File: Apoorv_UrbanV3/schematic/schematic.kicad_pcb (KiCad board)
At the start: 2 copper layers, 126 x 72 mm, 15 parts

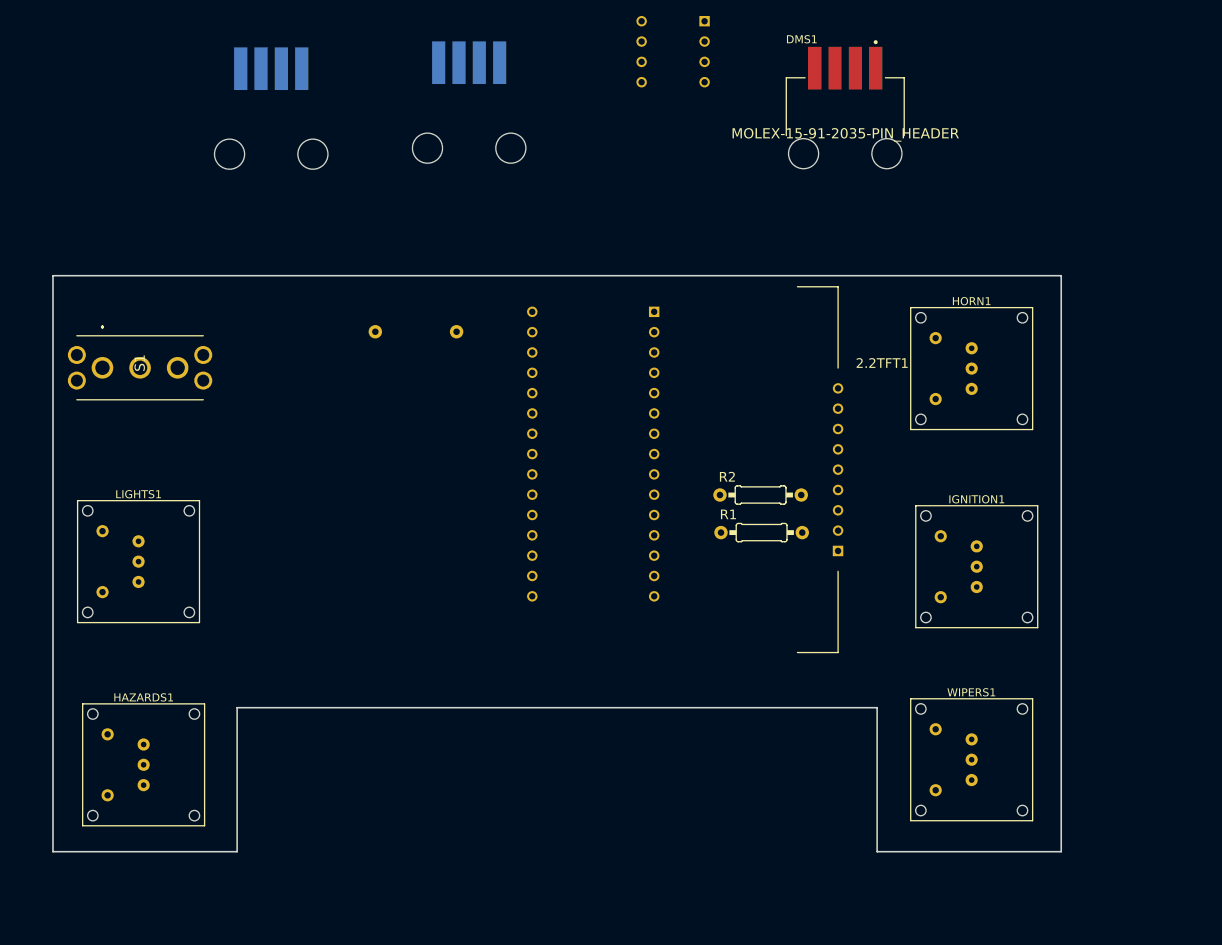
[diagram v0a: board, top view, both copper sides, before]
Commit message: ALMOST DONE, ROUTING LEFT
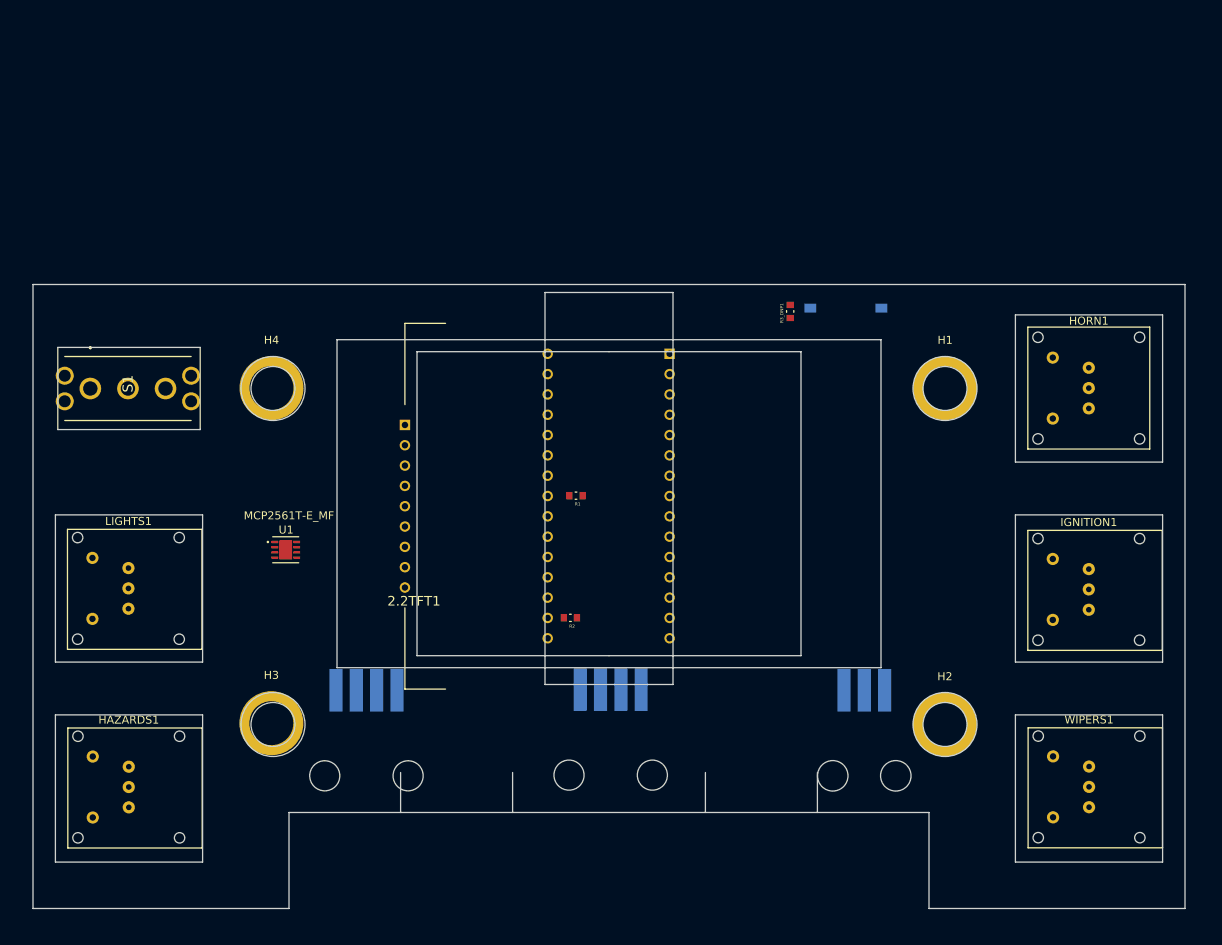
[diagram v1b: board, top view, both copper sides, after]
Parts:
- removed TRANSCEIVER1: MCP2561-THROUGH, schematic:DIP787W46P254L927H533Q8
- added H1: MountingHole_Pad, MountingHole:MountingHole_5mm_Pad, F.Cu at (196.1, 68.5)
- added H2: MountingHole_Pad, MountingHole:MountingHole_5mm_Pad, F.Cu at (196.0, 110.5)
- added H3: MountingHole_Pad, MountingHole:MountingHole_5mm_Pad, F.Cu at (111.9, 110.4)
- added H4: MountingHole_Pad, MountingHole:MountingHole_5mm_Pad, F.Cu at (111.9, 68.5)
- added S2: DS04-254-2-01BK-SMT, dip_swtich_1pos:SW_DS04-254-2-01BK-SMT, B.Cu at (183.7, 58.5)
- added U1: MCP2561T-E_MF, MCP2561:MCP2561T-E&slash_MF, F.Cu at (113.6, 88.7)
- DMS1: footprint eec:Molex-15-91-2045-0-0-0 -> 15-91-2035:15912035; moved to B.Cu
- R1, R2: footprint schematic:0207_10 -> 10k_resistor:RESC1608X55N
- R3_DNP1: footprint schematic:0207_10 -> 10k_resistor:RESC1608X55N; moved to F.Cu
- moved MAINPLUG1 88.5 mm to (154.3, 114.4)
- moved DMS1 80.3 mm to (186.0, 116.9), turned to 180 degrees
- moved BRAKE+THROTTLE1 79.5 mm to (123.7, 114.4)
- moved 2.2TFT1 49.3 mm to (131.1, 83.2), turned to 0 degrees
- moved R3_DNP1 46.8 mm to (176.7, 58.9), turned to 90 degrees
- moved R2 28.3 mm to (149.2, 97.2), turned to 180 degrees
- moved R1 23.7 mm to (149.9, 81.9), turned to 180 degrees
- moved WIPERS1 15.1 mm to (214.1, 113.2)
- moved HORN1 14.8 mm to (214.0, 63.4)
- moved IGNITION1 14.3 mm to (214.0, 88.6)
- moved STM32L432 5.59 mm to (154.0, 70.5)
- moved LIGHTS1 3.58 mm to (94.0, 88.4)
- moved HAZARDS1 3.34 mm to (94.0, 113.3)
- moved S1 3.00 mm to (89.2, 68.5)
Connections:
- 2.2TFT1 pad 4: +5V -> Net-(2.2TFT1-Pad4)
- 2.2TFT1 pad 5: Net-(2.2TFT1-Pad5) -> +5V
- R1 pad 2: +5V -> Net-(2.2TFT1-Pad4)
- R3_DNP1 pad 2: Net-(MAINPLUG1-Pad2) -> Net-(R3_DNP1-Pad2)
- STM32L432 pad 22: Net-(2.2TFT1-Pad5) -> +5V
- STM32L432 pad 23: +5V -> Net-(2.2TFT1-Pad4)
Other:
- board size 126 x 72 mm -> 144 x 78 mm
- board text removed: "ELEC_URB_STEERING_R3"
- board text removed: "SEMA"

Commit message: V3 done design review pending
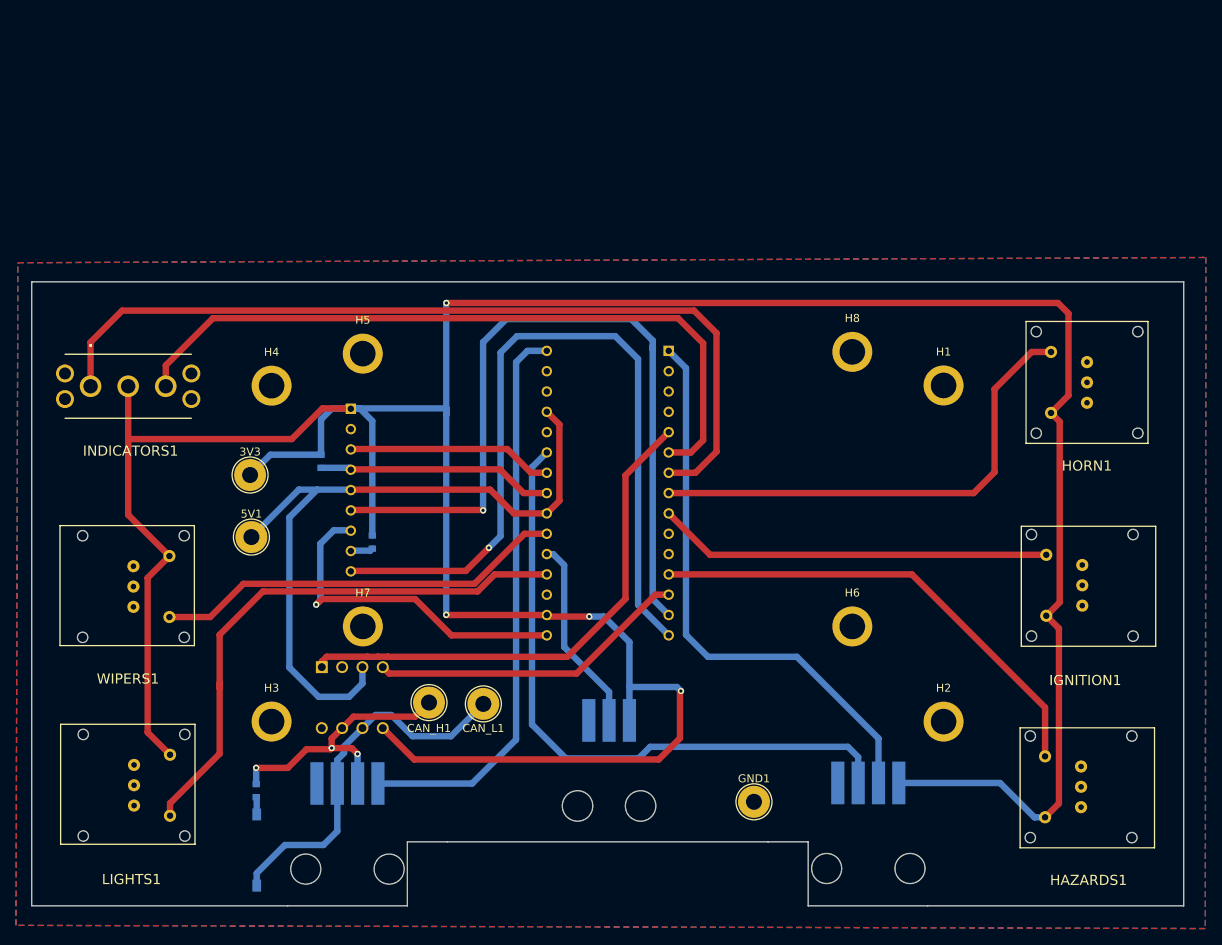
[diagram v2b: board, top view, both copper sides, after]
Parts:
- removed 2.2TFT1: 2.2TFT, schematic:2.2TFT
- removed U1: MCP2561T-E_MF, MCP2561:MCP2561T-E&slash_MF
- added 3V3: TestPoint, TestPoint:TestPoint_THTPad_D4.0mm_Drill2.0mm, F.Cu at (109.2, 79.3)
- added 5V1: TestPoint, TestPoint:TestPoint_THTPad_D4.0mm_Drill2.0mm, F.Cu at (109.4, 87.1)
- added CAN_H1: TestPoint, TestPoint:TestPoint_THTPad_D4.0mm_Drill2.0mm, F.Cu at (131.6, 107.8)
- added CAN_L1: TestPoint, TestPoint:TestPoint_THTPad_D4.0mm_Drill2.0mm, F.Cu at (138.4, 108.0)
- added CAN_TRNSVR1: `, footprints:MCP2562FD-H&slash_P, B.Cu at (118.2, 103.4)
- added GND1: TestPoint, TestPoint:TestPoint_THTPad_D4.0mm_Drill2.0mm, F.Cu at (172.2, 120.2)
- added H5: MountingHole_Pad, MountingHole:MountingHole_3.2mm_M3_Pad, F.Cu at (123.3, 64.2)
- added H6: MountingHole_Pad, MountingHole:MountingHole_3.2mm_M3_Pad, F.Cu at (184.5, 98.3)
- added H7: MountingHole_Pad, MountingHole:MountingHole_3.2mm_M3_Pad, F.Cu at (123.3, 98.3)
- added H8: MountingHole_Pad, MountingHole:MountingHole_3.2mm_M3_Pad, F.Cu at (184.5, 63.9)
- added LCD1: 2.2TFT, schematic:2.2TFT, F.Cu at (124.3, 81.2)
- BRAKE+THROTTLE1: value MOLEX-15-91-2045-PIN_HEADER -> `
- DMS1: value MOLEX-15-91-2035-PIN_HEADER -> `
- H1, H2, H3, H4: footprint MountingHole:MountingHole_5mm_Pad -> MountingHole:MountingHole_3.2mm_M3_Pad
- HAZARDS1, IGNITION1, LIGHTS1, WIPERS1: value LP11EE1NCSYG -> `
- HORN1: value LP11OA1TCSYY -> `
- INDICATORS1: renamed from S1; value M2013TXG13-DA -> `
- R1, R2: moved to B.Cu
- R_CAN1: renamed from R3_DNP1; moved to B.Cu
- S_CAN1: renamed from S2; value DS04-254-2-01BK-SMT -> ~
- moved WIPERS1 120.4 mm to (94.6, 98.4), turned to 180 degrees
- moved HAZARDS1 119.0 mm to (213.1, 113.2)
- moved S_CAN1 100.1 mm to (110.0, 126.2), turned to 270 degrees
- moved R_CAN1 89.7 mm to (110.0, 118.8), turned to 270 degrees
- moved BRAKE+THROTTLE1 63.8 mm to (186.5, 126.0)
- moved MAINPLUG1 34.9 mm to (121.4, 126.1)
- moved LIGHTS1 34.8 mm to (94.7, 123.2), turned to 180 degrees
- moved R1 32.2 mm to (118.1, 77.6), turned to 270 degrees
- moved DMS1 32.1 mm to (154.1, 120.7)
- moved R2 26.5 mm to (124.5, 87.7), turned to 270 degrees
- moved IGNITION1 0.96 mm to (213.2, 88.1)
- moved HORN1 0.74 mm to (213.8, 62.7)
- moved H2 0.40 mm to (195.9, 110.2)
- moved H1 0.39 mm to (195.9, 68.2)
- moved STM32L432 0.38 mm to (153.9, 70.2)
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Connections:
- net +5V renamed LCD_DC
- net Net-(2.2TFT1-Pad4) renamed LCD_RST
- net Net-(DMS1-Pad2) renamed DMS
- net Net-(HAZARDS1-Pad2) renamed HAZARDS
- net Net-(HORN1-Pad2) renamed HORN
- net Net-(IGNITION1-Pad2) renamed IGNITION
- net Net-(LIGHTS1-Pad2) renamed LIGHTS
- net Net-(MAINPLUG1-Pad2) renamed CAN_L
- net Net-(MAINPLUG1-Pad3) renamed CAN_H
- net Net-(S1-PadLEFT) renamed IND_LEFT
- net Net-(S1-PadRIGHT) renamed IND_RIGHT
- net Net-(STM32L432-Pad21) renamed WIPRERS
- R2 pad 2: Net-(2.2TFT1-Pad8) -> LCD_LED
- STM32L432 pad 13: Net-(STM32L432-Pad13) -> RXD
- STM32L432 pad 14: Net-(2.2TFT1-Pad6) -> LCD_MOSI
- STM32L432 pad 15: Net-(2.2TFT1-Pad9) -> LCD_MISO
- STM32L432 pad 16: Net-(2.2TFT1-Pad7) -> LCD_SCK
- STM32L432 pad 24: Net-(2.2TFT1-Pad3) -> LCD_CS
- STM32L432 pad 5: Net-(STM32L432-Pad5) -> TXD
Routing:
- net +3V3: track 0.00 -> 419.3 mm, vias 0 -> 4
- net IND_LEFT: track 0.00 -> 108.4 mm
- net LCD_MISO: track 0.00 -> 98.9 mm, vias 0 -> 1
- net LCD_MOSI: track 0.00 -> 96.8 mm, vias 0 -> 1
- net LCD_DC: track 0.00 -> 91.7 mm
- net IND_RIGHT: track 0.00 -> 90.6 mm
- net Net-(BRAKE+THROTTLE1-Pad2): track 0.00 -> 81.7 mm
- net Net-(BRAKE+THROTTLE1-Pad3): track 0.00 -> 71.4 mm
- net +12V: track 0.00 -> 71.1 mm
- net LIGHTS: track 0.00 -> 69.8 mm
- net TXD: track 0.00 -> 65.0 mm
- net HORN: track 0.00 -> 61.2 mm
- net HAZARDS: track 0.00 -> 60.0 mm
- net WIPRERS: track 0.00 -> 51.5 mm
- net IGNITION: track 0.00 -> 49.3 mm
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- added copper zone on B.Cu, net GND
- added copper zone on F.Cu, net GND
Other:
- outline, holes or cut-outs redrawn
- rule trace_min: 0.1524 -> 0.13
